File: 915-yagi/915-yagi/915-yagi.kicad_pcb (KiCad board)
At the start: 2 copper layers, 175 x 171.5 mm, 1 part, among them J1 Conn_Coaxial

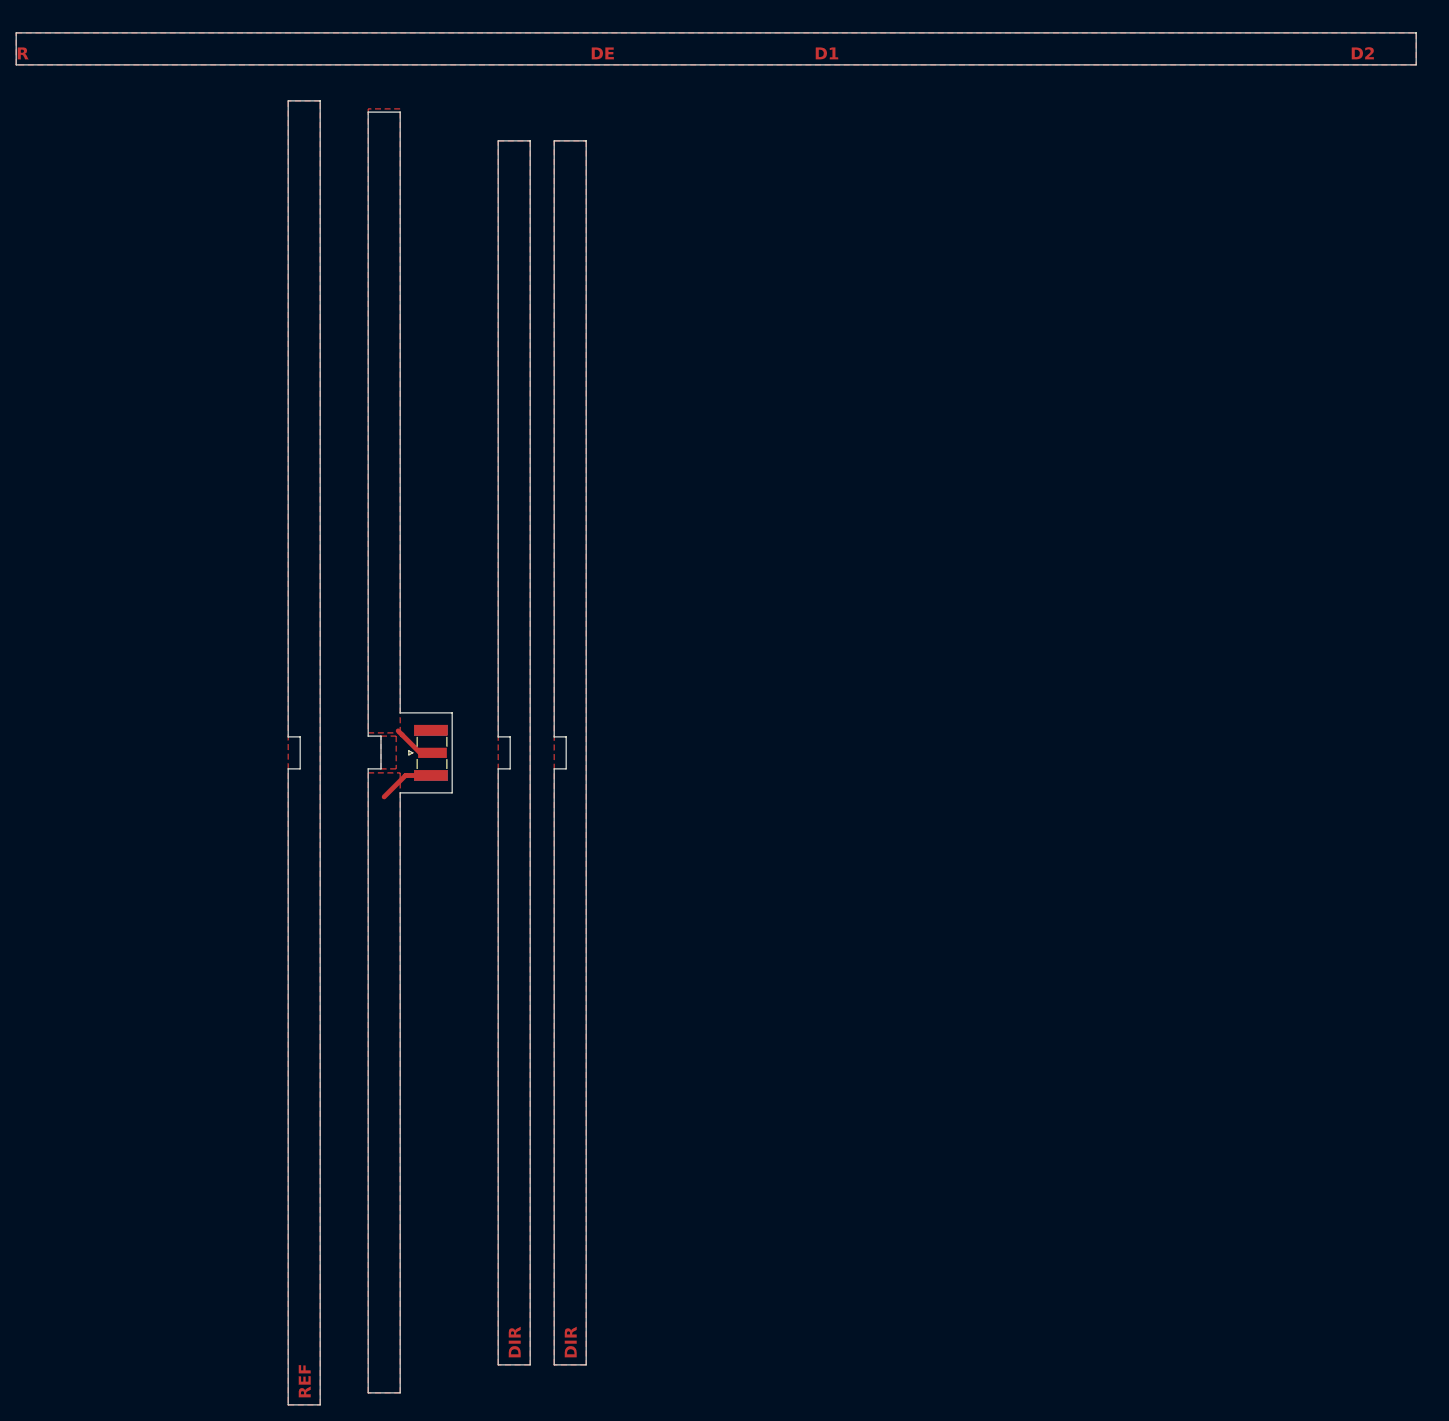
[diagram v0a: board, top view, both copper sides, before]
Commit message: updates
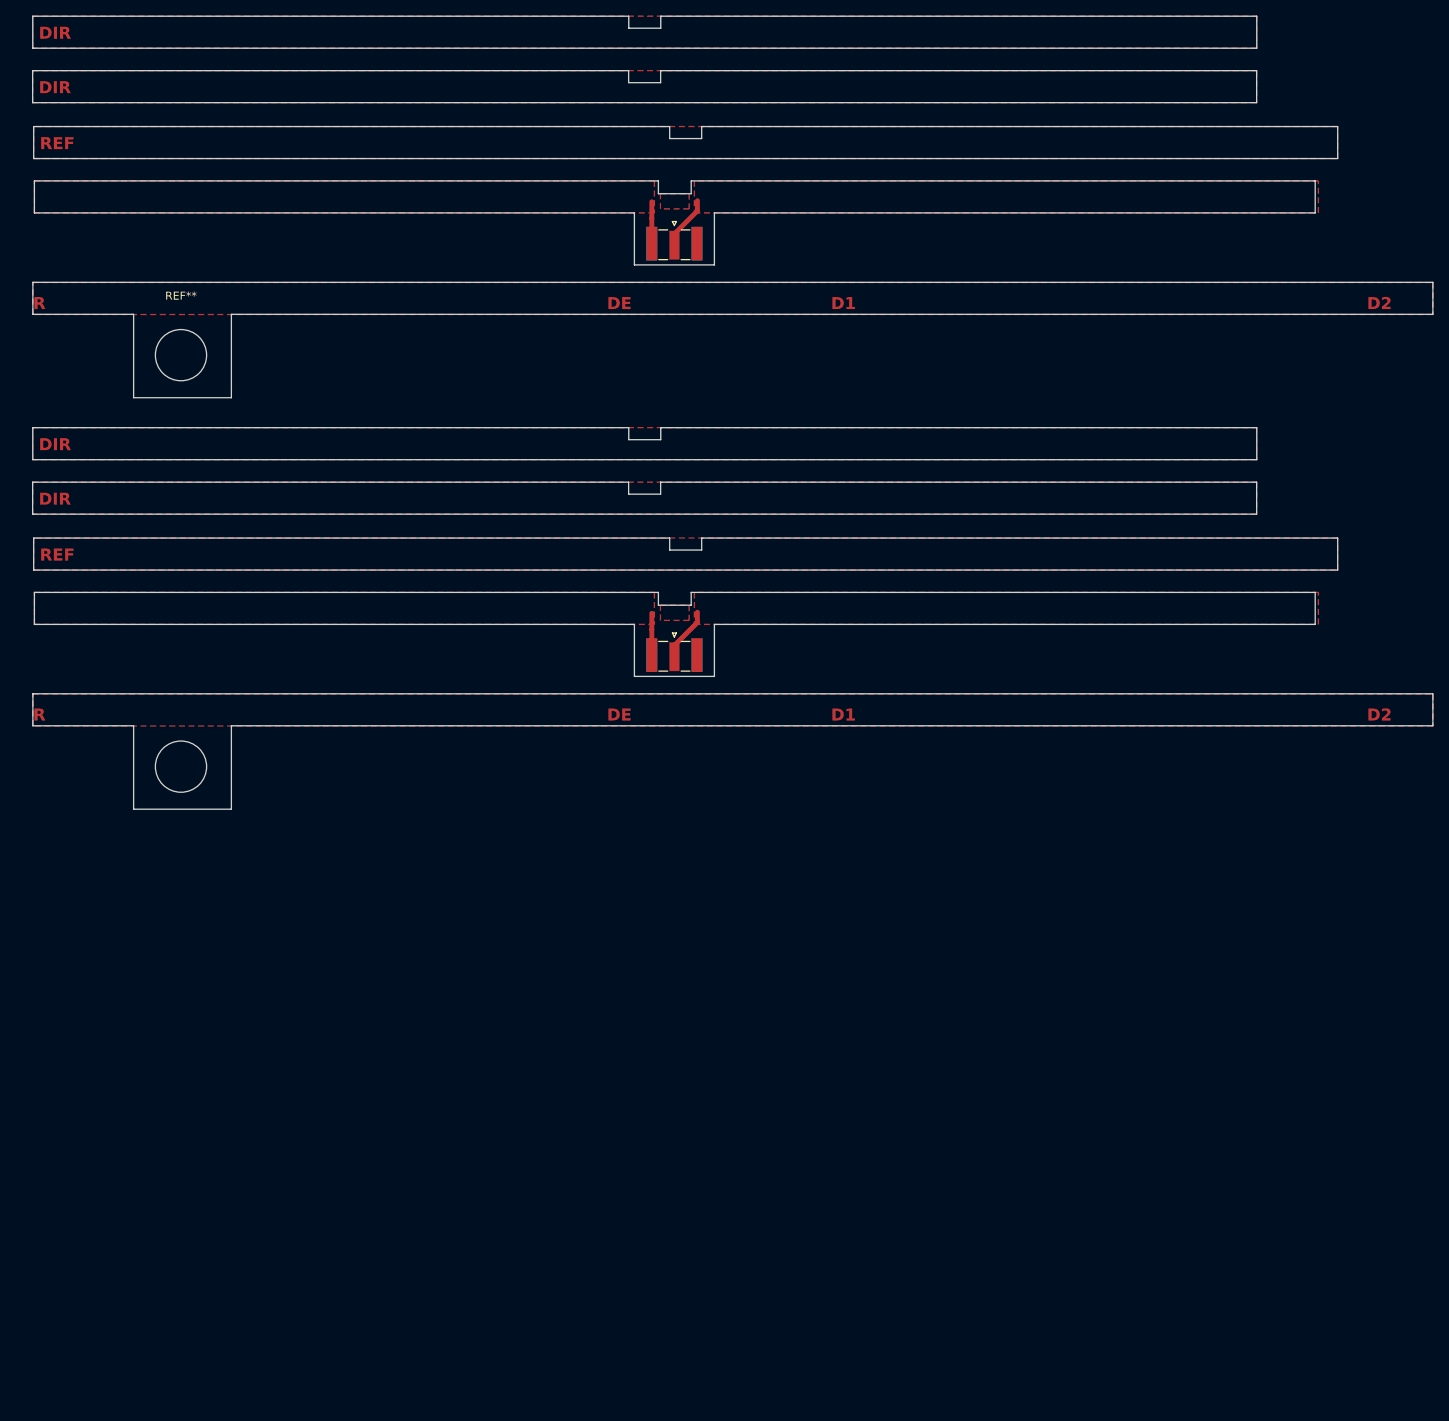
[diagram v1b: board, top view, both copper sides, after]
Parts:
- removed the J1 at (69.3, 107.5)
- added ?: , , F.Cu at (38.1, 109.2)
- added J1: Conn_Coaxial, Connector_Coaxial:SMA_Samtec_SMA-J-P-X-ST-EM1_EdgeMount, F.Cu at (99.8, 43.8)
- added J1: Conn_Coaxial, Connector_Coaxial:SMA_Samtec_SMA-J-P-X-ST-EM1_EdgeMount, F.Cu at (99.8, 95.3)
- added REF**: MountingHole_6.4mm_M6, MountingHole:MountingHole_6.4mm_M6, F.Cu at (38.1, 57.8)
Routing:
- net ANT: track 5.43 -> 10.7 mm
- net GND: track 6.95 -> 10.5 mm
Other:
- board size 175 x 171.5 mm -> 175 x 99.1 mm
